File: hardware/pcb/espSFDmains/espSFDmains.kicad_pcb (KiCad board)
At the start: 4 copper layers, 124.5 x 63.5 mm, 80 parts, among them J1 Mains, J10 D1 & D2, J11 D3 & D4, J2 Mains Motor, J3 VDD, J4 D5 & D6, J5 Motor, J8 SFD Bus, J9 SFD Bus, U1 TXS0102DCT, U2 LM2675M-3.3, U3 WEMOS_D1_mini, U4 NCP1117-5.0_SOT223, U5 DS3231MZ

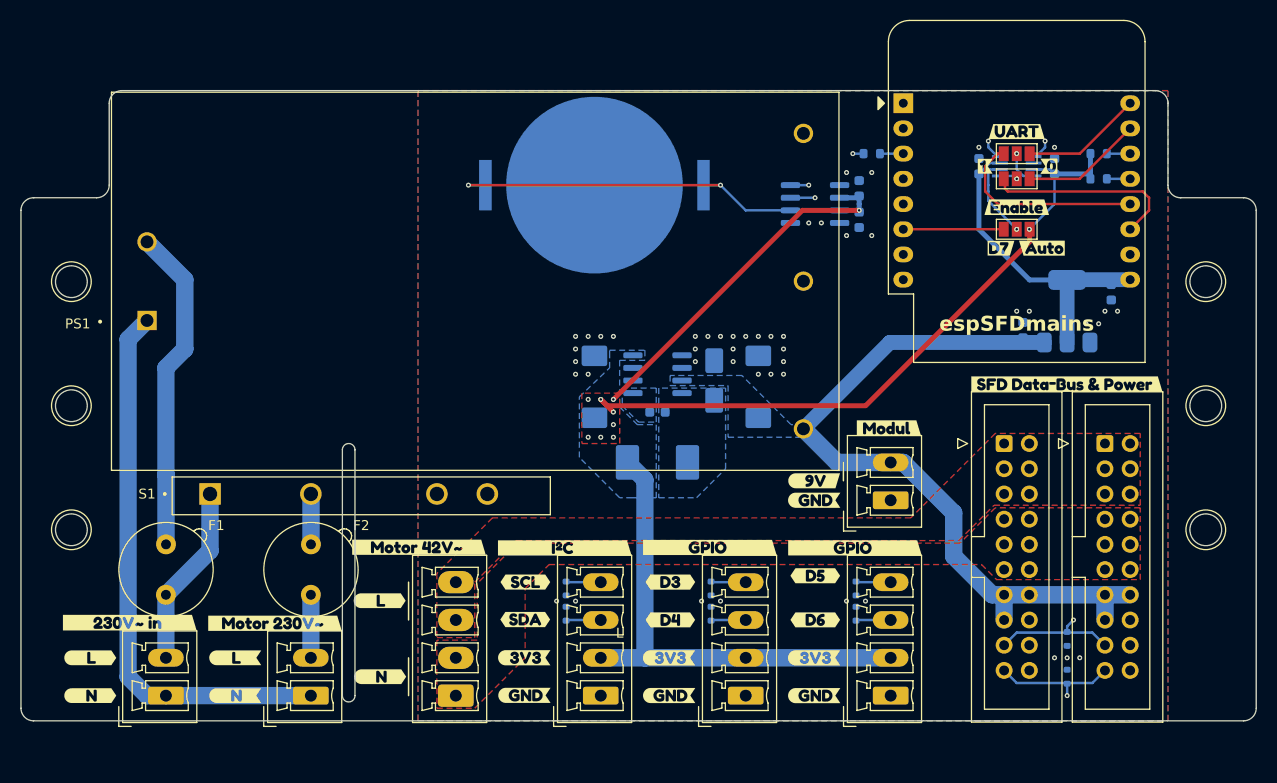
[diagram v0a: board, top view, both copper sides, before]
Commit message: bxcbxc
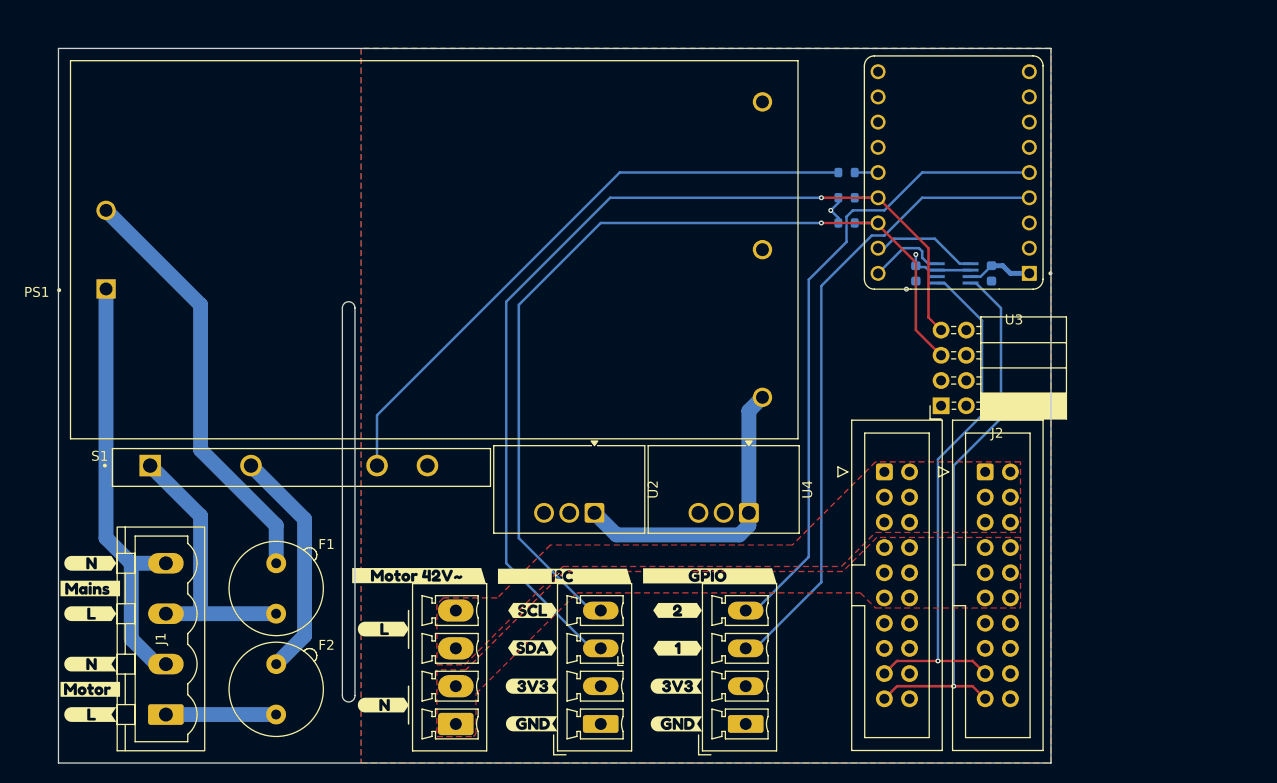
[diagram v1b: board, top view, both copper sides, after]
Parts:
- removed BT1: Battery_Cell, Battery:BatteryHolder_Keystone_3034_1x20mm
- removed C1: 15µF/50V, Capacitor_Tantalum_SMD:CP_EIA-7343-43_Kemet-X
- removed C2: 10nF/50V, Capacitor_SMD:C_0603_1608Metric
- removed C3: 68µF/16V, Capacitor_Tantalum_SMD:CP_EIA-7343-43_Kemet-X
- removed C6: 100nF/50V, Capacitor_SMD:C_0603_1608Metric
- removed C7: 1µF/50V, Capacitor_SMD:C_0603_1608Metric
- removed C8, C9: 10µF/25V, Capacitor_SMD:C_0603_1608Metric
- removed D1: SS14, Diode_SMD:D_SMA
- removed D2, D3, D4, D5, D6, D7, D8, D9: LESD5D5.0CT1G, Diode_SMD:D_SOD-523
- removed DRA1, DRA2: DIN_Rail_Adapter, MountingEquipment:DINRailAdapter_3xM3_PhoenixContact_1201578
- removed J3: VDD, Connector_Phoenix_MC:PhoenixContact_MCV_1,5_2-G-3.81_1x02_P3.81mm_Vertical
- removed J4: D5 & D6, Connector_Phoenix_MC:PhoenixContact_MCV_1,5_4-G-3.81_1x04_P3.81mm_Vertical
- removed JP1, JP5: RX Select, Jumper:SolderJumper-3_P1.3mm_Open_Pad1.0x1.5mm
- removed JP2: TX Select, Jumper:SolderJumper-3_P1.3mm_Open_Pad1.0x1.5mm
- removed L1: 33µH, Inductor_SMD:L_Chilisin_BMRB00060650
- removed U5: DS3231MZ, Package_SO:SOIC-8_3.9x4.9mm_P1.27mm
- removed kibuzzard-6985EF84: G***, kibuzzard-6985EF84
- removed kibuzzard-6985EF8A: G***, kibuzzard-6985EF8A
- removed kibuzzard-6985F394: G***, kibuzzard-6985F394
- removed kibuzzard-6985F472: G***, kibuzzard-6985F472
- removed kibuzzard-6985F4E1: G***, kibuzzard-6985F4E1
- removed kibuzzard-6985F4F7: G***, kibuzzard-6985F4F7
- removed kibuzzard-6985F567: G***, kibuzzard-6985F567
- removed kibuzzard-6985F5B0: G***, kibuzzard-6985F5B0
- removed kibuzzard-6985F603: G***, kibuzzard-6985F603
- removed kibuzzard-6985F68A: G***, kibuzzard-6985F68A
- removed the kibuzzard-699C2E08 at (108.5, 137.8)
- removed kibuzzard-699C2E8F: G***, kibuzzard-699C2E8F
- removed kibuzzard-699C2EC2: G***, kibuzzard-699C2EC2
- removed kibuzzard-699C2F1B: G***, kibuzzard-699C2F1B
- removed kibuzzard-699C2F31: G***, kibuzzard-699C2F31
- removed kibuzzard-699C2F5C: G***, kibuzzard-699C2F5C
- removed kibuzzard-699C2F61: G***, kibuzzard-699C2F61
- removed kibuzzard-699C2F67: G***, kibuzzard-699C2F67
- removed kibuzzard-699C2F70: G***, kibuzzard-699C2F70
- removed kibuzzard-699C2F7D: G***, kibuzzard-699C2F7D
- removed kibuzzard-699C2F83: G***, kibuzzard-699C2F83
- removed kibuzzard-699C2F89: G***, kibuzzard-699C2F89
- removed kibuzzard-699C2F8F: G***, kibuzzard-699C2F8F
- removed kibuzzard-699C2F95: G***, kibuzzard-699C2F95
- removed kibuzzard-699C2F9C: G***, kibuzzard-699C2F9C
- removed kibuzzard-699C2FA4: G***, kibuzzard-699C2FA4
- removed kibuzzard-699C2FB0: G***, kibuzzard-699C2FB0
- added kibuzzard-69B3E2B0: G***, kibuzzard-69B3E2B0, F.Cu at (31.4, 152.1)
- added kibuzzard-69B3E2CA: G***, kibuzzard-69B3E2CA, F.Cu at (31.4, 141.9)
- added kibuzzard-69B3E350: G***, kibuzzard-69B3E350, F.Cu at (61.0, 146.0)
- added kibuzzard-69B3E357: G***, kibuzzard-69B3E357, F.Cu at (61.0, 153.7)
- added kibuzzard-69B3E35C: G***, kibuzzard-69B3E35C, F.Cu at (76.0, 144.1)
- added kibuzzard-69B3E365: G***, kibuzzard-69B3E365, F.Cu at (76.0, 147.9)
- added kibuzzard-69B3E36A: G***, kibuzzard-69B3E36A, F.Cu at (75.9, 151.8)
- added kibuzzard-69B3E36E: G***, kibuzzard-69B3E36E, F.Cu at (75.9, 155.5)
- added kibuzzard-69B3E379: G***, kibuzzard-69B3E379, F.Cu at (90.6, 144.1)
- added kibuzzard-69B3E37F: G***, kibuzzard-69B3E37F, F.Cu at (90.6, 147.9)
- added kibuzzard-69B3E384: G***, kibuzzard-69B3E384, F.Cu at (90.5, 151.8)
- added kibuzzard-69B3E389: G***, kibuzzard-69B3E389, F.Cu at (90.5, 155.6)
- C4, C5: value 100nF/50V -> 100nF/25V
- J1: footprint Connector_Phoenix_MC:PhoenixContact_MCV_1,5_2-G-3.81_1x02_P3.81mm_Vertical -> Connector_Phoenix_MSTB:PhoenixContact_MSTBVA_2,5_4-G-5,08_1x04_P5.08mm_Vertical
- J2: value Mains Motor -> Conn_02x04_Odd_Even; footprint Connector_Phoenix_MC:PhoenixContact_MCV_1,5_2-G-3.81_1x02_P3.81mm_Vertical -> Connector_PinSocket_2.54mm:PinSocket_2x04_P2.54mm_Horizontal
- R3: value 100R -> 330R
- U2: value LM2675M-3.3 -> TSR3-2433N; footprint Package_SO:SOIC-8_3.9x4.9mm_P1.27mm -> Converter_DCDC:Converter_DCDC_TRACO_TSR2-24xxN_TSR2-24xxxN_THT; moved to F.Cu
- U3: value WEMOS_D1_mini -> ESP32-S3-ZERO; footprint RF_Module:WEMOS_D1_mini_light -> lib:ESP32-S3-ZERO
- U4: value NCP1117-5.0_SOT223 -> TSR3-2450N; footprint Package_TO_SOT_SMD:SOT-223-3_TabPin2 -> Converter_DCDC:Converter_DCDC_TRACO_TSR2-24xxN_TSR2-24xxxN_THT; moved to F.Cu
- moved J2 69.9 mm to (117.2, 123.5), turned to 180 degrees
- moved U4 38.0 mm to (97.8, 134.3), turned to -90 degrees
- moved R4 26.3 mm to (107.6, 105.1)
- moved R5 25.5 mm to (107.6, 102.5)
- moved C5 17.7 mm to (114.6, 110.2), turned to 90 degrees
- moved kibuzzard-699C2EF8 15.7 mm to (31.4, 154.6)
- moved U2 15.3 mm to (82.2, 134.3), turned to -90 degrees
- moved kibuzzard-699C2F02 14.9 mm to (31.4, 149.5)
- moved kibuzzard-6985EF62 13.3 mm to (31.4, 139.4)
- moved F2 12.6 mm to (50.2, 154.6)
- moved U1 12.5 mm to (118.4, 110.2), turned to 0 degrees
- moved J8 12.4 mm to (111.4, 130.2)
- moved J9 12.4 mm to (121.6, 130.2)
- moved F1 11.3 mm to (50.2, 144.5)
- moved C4 10.9 mm to (122.2, 110.2), turned to 90 degrees
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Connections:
- J1 pad 1: NEUT -> 230V Motor
- J1 pad 2: LINE -> NEUT
- J10 pad 3: D2/SDA -> SDA
- J10 pad 4: D1/SCL -> SCL
- J11 pad 3: D4/RX1 -> GPIO1
- J11 pad 4: D3/TX1 -> GPIO2
- J2 pad 1: NEUT -> +9V
- J2 pad 2: 230V Motor -> +9V
- R4 pad 2: D1/SCL -> SCL
- R5 pad 2: D2/SDA -> SDA
- U1 pad 4: TX Selected -> TX_
- U1 pad 5: RX Selected -> RX_
- U1 pad 6: OE -> +3.3V
- U2 pad 1: /CB -> +9V
- U2 pad 2: unconnected-(U2-NC-Pad2) -> GND
- U2 pad 3: unconnected-(U2-NC-Pad3) -> +3.3V
- U3 pad 1: unconnected-(U3-~{RST}-Pad1) -> GPIO1
- U3 pad 10: GND -> unconnected-(U3-GP10-Pad10)
- U3 pad 11: D4/RX1 -> En Motor
- U3 pad 12: D3/TX1 -> SDA
- U3 pad 13: D2/SDA -> SCL
- U3 pad 2: unconnected-(U3-A0-Pad2) -> GPIO2
- U3 pad 3: En Motor -> unconnected-(U3-GP3-Pad3)
- U3 pad 4: D5 -> unconnected-(U3-GP4-Pad4)
- U3 pad 5: D6 -> unconnected-(U3-GP5-Pad5)
- U3 pad 6: Enable UART -> unconnected-(U3-GP6-Pad6)
- U3 pad 9: +5V -> unconnected-(U3-GP9-Pad9)
- U4 pad 1: GND -> +9V
- U4 pad 2: +5V -> GND
- U4 pad 3: +9V -> +5V
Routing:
- net +3.3V: track 154.5 -> 10.00 mm, vias 10 -> 2
- net SDA: track 0.00 -> 99.5 mm, vias 0 -> 1
- net D2/SDA: track 93.5 -> 0.00 mm, vias 1 -> 0
- net SCL: track 0.00 -> 92.7 mm, vias 0 -> 1
- net D1/SCL: track 91.2 -> 0.00 mm, vias 1 -> 0
- net D4/RX1: track 84.0 -> 0.00 mm
- net D3/TX1: track 82.7 -> 0.00 mm
- net GPIO1: track 0.00 -> 64.9 mm
- net GPIO2: track 0.00 -> 64.7 mm
- net D6: track 51.3 -> 0.00 mm
- net D5: track 48.4 -> 0.00 mm
- net Net-(BT1-+): track 36.9 -> 0.00 mm, vias 2 -> 0
- net +9V: track 75.4 -> 48.7 mm
- net +5V: track 31.8 -> 55.2 mm
- net RX: track 76.0 -> 55.4 mm, vias 2 -> 1
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- added copper zone on In1.Cu, net +3.3V
- added copper zone on In1.Cu, net +9V
- removed copper zone on B.Cu, net +3.3V
- removed copper zone on F.Cu, net +3.3V
- removed copper zone on B.Cu, net +9V
- removed copper zone on B.Cu, net /CB
- removed copper zone on B.Cu, net /VSW
- removed copper zone on In1.Cu, net GND
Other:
- board size 124.5 x 63.5 mm -> 100 x 72 mm
- board text removed: "espSFDmains"
